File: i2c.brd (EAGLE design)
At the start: 100 x 80 mm, 7 parts, among them IC1 24LC024SN, IC2 24LC024ST, X1 2510-

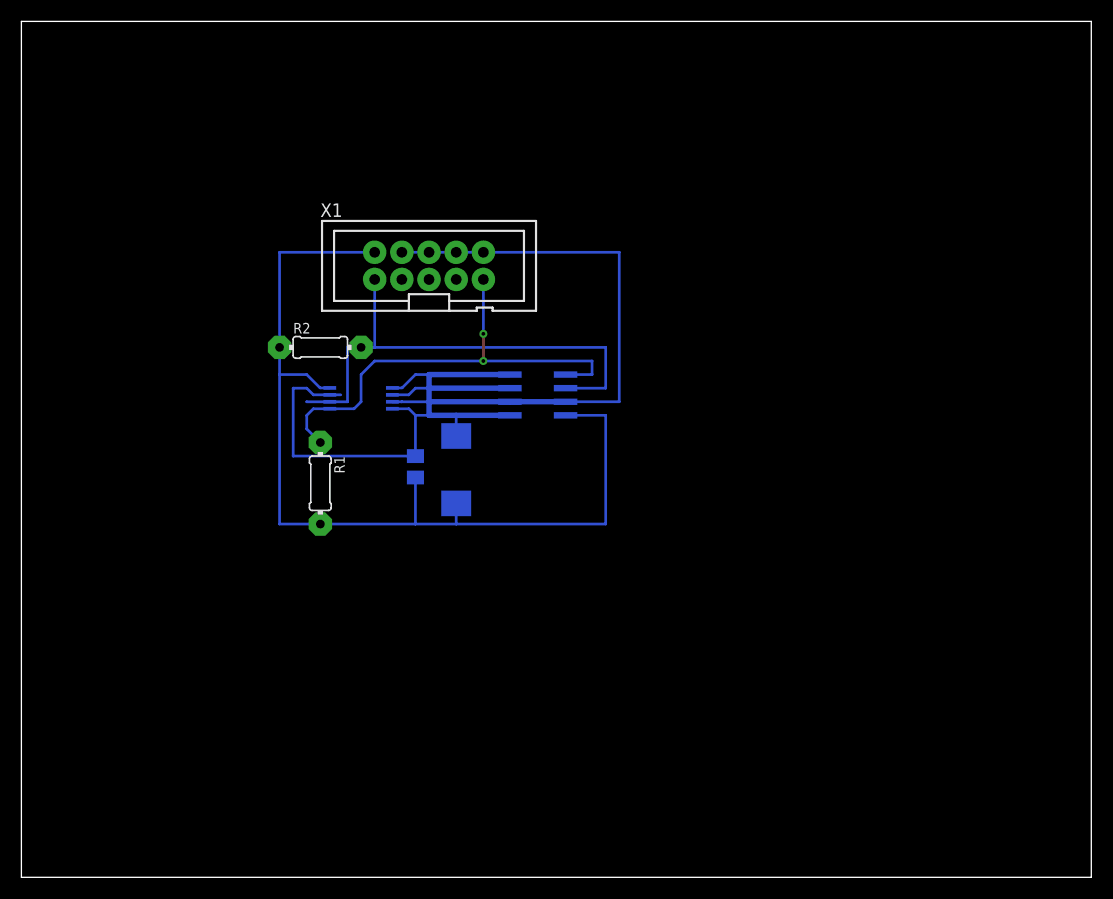
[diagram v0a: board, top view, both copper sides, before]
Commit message: Черновой вариант с заливкой
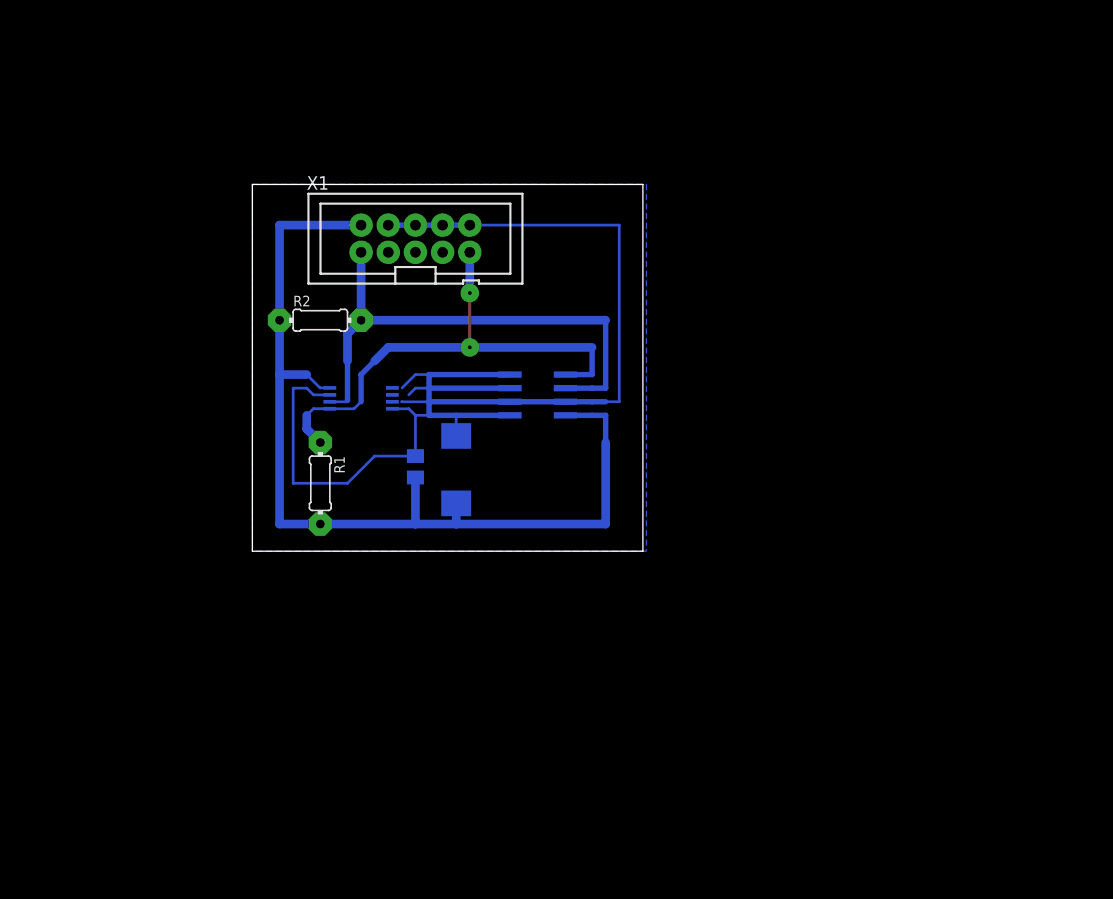
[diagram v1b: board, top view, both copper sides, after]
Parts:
- moved X1 2.84 mm to (36.8, 59.7)
- moved R2 2.54 mm to (27.9, 52.1)
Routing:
- net MISO: track 44.7 -> 49.7 mm
- net GND: track 121.6 -> 124.6 mm
- net MOSI: track 46.9 -> 49.0 mm
- net VCC: track 90.2 -> 91.4 mm
- added copper zone on layer 16, net GND
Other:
- board size 100 x 80 mm -> 36.5 x 34.3 mm
